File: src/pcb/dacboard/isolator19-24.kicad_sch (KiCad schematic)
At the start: 18 parts, among them U101 ISO7761FQDBQRQ1, U102 ISO7761FQDBQRQ1, U103 ISO7761FQDBQRQ1, U104 ISO7761FQDBQRQ1, U105 ISO7761FQDBQRQ1, U106 ISO7761FQDBQRQ1

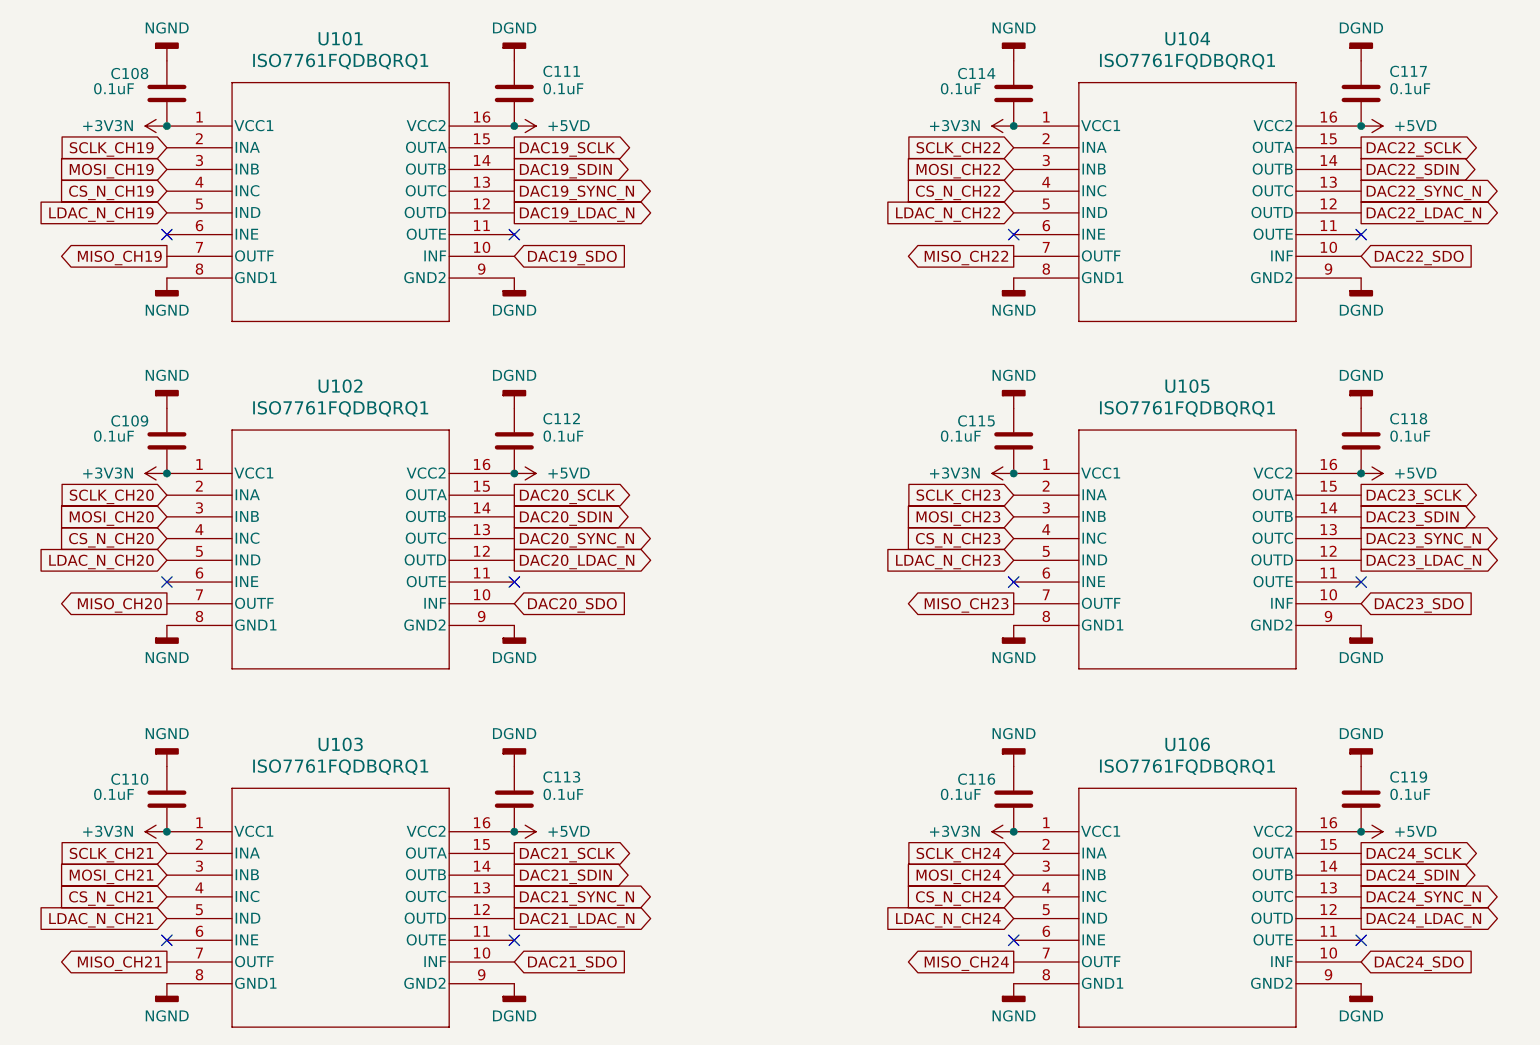
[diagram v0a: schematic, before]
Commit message: dacboard routing
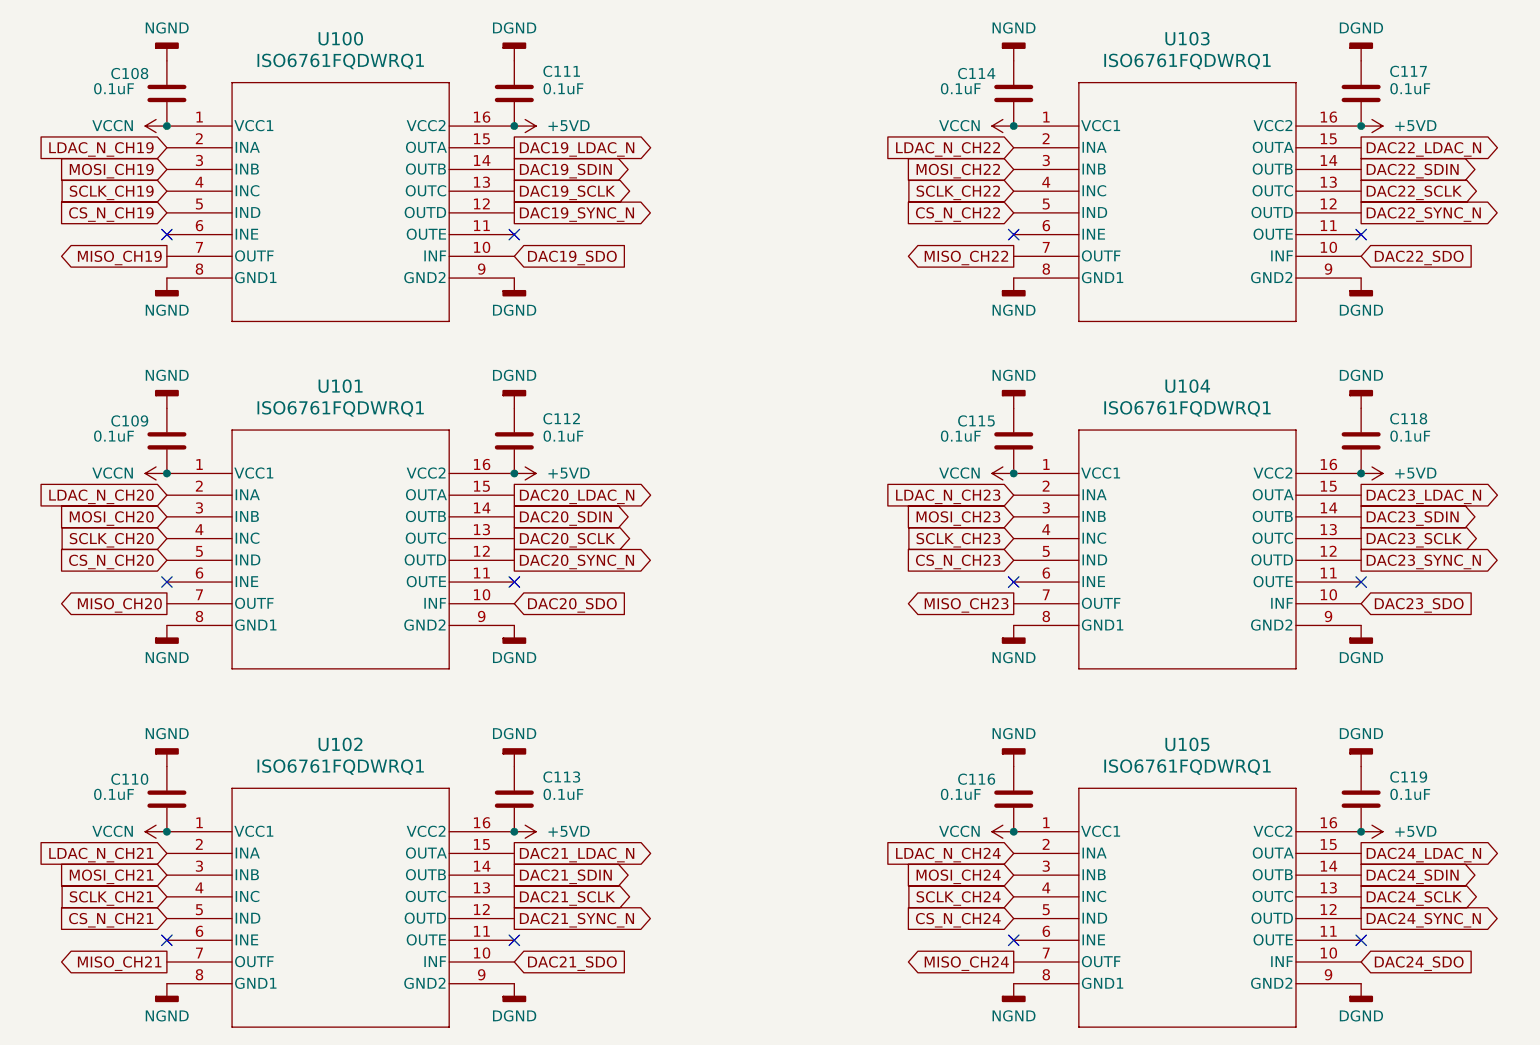
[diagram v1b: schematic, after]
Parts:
- removed U101, U102, U103, U104, U105, U106: ISO7761FQDBQRQ1, DBQ16_TEX, symbol 2025-11-18_20-36-36:ISO7761FQDBQRQ1
- added U100, U101, U102, U103, U104, U105: ISO6761FQDWRQ1, ISO6761:SOIC16_DW_TEX, symbol 2025-11-20_00-47-15:ISO6761FQDWRQ1
- C108, C109, C110, C111, C112, C113, C114, C115, C116, C117, C118, C119: footprint (none) -> Capacitor_SMD:C_0402_1005Metric_Pad0.74x0.62mm_HandSolder
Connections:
- net +5VD: now also U100.16 (VCC2), U101.16 (VCC2), U102.16 (VCC2), U103.16 (VCC2), U104.16 (VCC2), U105.16 (VCC2)
- net CS_N_CH19: now also U100.5 (IND)
- net CS_N_CH20: now also U101.5 (IND)
- net CS_N_CH21: now also U102.5 (IND)
- net CS_N_CH22: now also U103.5 (IND)
- net CS_N_CH23: now also U104.5 (IND)
- net CS_N_CH24: now also U105.5 (IND)
- net DAC19_LDAC_N: now also U100.15 (OUTA)
- net DAC19_SCLK: now also U100.13 (OUTC)
- net DAC19_SDIN: now also U100.14 (OUTB)
- net DAC19_SDO: now also U100.10 (INF)
- net DAC19_SYNC_N: now also U100.12 (OUTD)
- net DAC20_LDAC_N: now also U101.15 (OUTA)
- net DAC20_SCLK: now also U101.13 (OUTC)
- net DAC20_SDIN: now also U101.14 (OUTB)
- net DAC20_SDO: now also U101.10 (INF)
- net DAC20_SYNC_N: now also U101.12 (OUTD)
- net DAC21_LDAC_N: now also U102.15 (OUTA)
- net DAC21_SCLK: now also U102.13 (OUTC)
- net DAC21_SDIN: now also U102.14 (OUTB)
- net DAC21_SDO: now also U102.10 (INF)
- net DAC21_SYNC_N: now also U102.12 (OUTD)
- net DAC22_LDAC_N: now also U103.15 (OUTA)
- net DAC22_SCLK: now also U103.13 (OUTC)
- net DAC22_SDIN: now also U103.14 (OUTB)
- net DAC22_SDO: now also U103.10 (INF)
- net DAC22_SYNC_N: now also U103.12 (OUTD)
- net DAC23_LDAC_N: now also U104.15 (OUTA)
- net DAC23_SCLK: now also U104.13 (OUTC)
- net DAC23_SDIN: now also U104.14 (OUTB)
- net DAC23_SDO: now also U104.10 (INF)
- net DAC23_SYNC_N: now also U104.12 (OUTD)
- net DAC24_LDAC_N: now also U105.15 (OUTA)
- net DAC24_SCLK: now also U105.13 (OUTC)
- net DAC24_SDIN: now also U105.14 (OUTB)
- net DAC24_SDO: now also U105.10 (INF)
- net DAC24_SYNC_N: now also U105.12 (OUTD)
- net DGND: now also U100.9 (GND2), U101.9 (GND2), U102.9 (GND2), U103.9 (GND2), U104.9 (GND2), U105.9 (GND2)
- net LDAC_N_CH19: now also U100.2 (INA)
- net LDAC_N_CH20: now also U101.2 (INA)
- net LDAC_N_CH21: now also U102.2 (INA)
- net LDAC_N_CH22: now also U103.2 (INA)
- net LDAC_N_CH23: now also U104.2 (INA)
- net LDAC_N_CH24: now also U105.2 (INA)
- net MISO_CH19: now also U100.7 (OUTF)
- net MISO_CH20: now also U101.7 (OUTF)
- net MISO_CH21: now also U102.7 (OUTF)
- net MISO_CH22: now also U103.7 (OUTF)
- net MISO_CH23: now also U104.7 (OUTF)
- net MISO_CH24: now also U105.7 (OUTF)
- net MOSI_CH19: now also U100.3 (INB)
- net MOSI_CH20: now also U101.3 (INB)
- net MOSI_CH21: now also U102.3 (INB)
- net MOSI_CH22: now also U103.3 (INB)
- net MOSI_CH23: now also U104.3 (INB)
- net MOSI_CH24: now also U105.3 (INB)
- net NGND: now also U100.8 (GND1), U101.8 (GND1), U102.8 (GND1), U103.8 (GND1), U104.8 (GND1), U105.8 (GND1)
- net SCLK_CH19: now also U100.4 (INC)
- net SCLK_CH20: now also U101.4 (INC)
- net SCLK_CH21: now also U102.4 (INC)
- net SCLK_CH22: now also U103.4 (INC)
- net SCLK_CH23: now also U104.4 (INC)
- net SCLK_CH24: now also U105.4 (INC)
- net +3V3N renamed VCCN
- net VCCN: now also U100.1 (VCC1), U101.1 (VCC1), U102.1 (VCC1), U103.1 (VCC1), U104.1 (VCC1), U105.1 (VCC1)
